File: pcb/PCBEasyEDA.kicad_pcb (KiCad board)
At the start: 2 copper layers, 63.4 x 89 mm, 56 parts

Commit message: YAY
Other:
- board text removed: "#10: Error: unsupported layer id: 100 found in CIRCLE (gge2481) of gge9d629947a8bba335; circle ignored"
- board text removed: "#11: Error: unsupported layer id: 100 found in CIRCLE (gge2484) of gge9d629947a8bba335; circle ignored"
- board text removed: "#12: Error: unsupported layer id: 100 found in CIRCLE (gge2487) of gge9d629947a8bba335; circle ignored"
- board text removed: "#13: Error: unsupported layer id: 100 found in CIRCLE (gge2490) of gge9d629947a8bba335; circle ignored"
- board text removed: "#14: Error: unsupported layer id: 100 found in CIRCLE (gge2493) of gge9d629947a8bba335; circle ignored"
- board text removed: "#15: Error: unsupported layer id: 100 found in CIRCLE (gge2496) of gge9d629947a8bba335; circle ignored"
- board text removed: "#16: Error: unsupported layer id: 100 found in CIRCLE (gge2499) of gge9d629947a8bba335; circle ignored"
- board text removed: "#17: Error: unsupported layer id: 100 found in CIRCLE (gge2502) of gge9d629947a8bba335; circle ignored"
- board text removed: "#18: Error: unsupported layer id: 100 found in CIRCLE (gge2505) of gge9d629947a8bba335; circle ignored"
- board text removed: "#19: Error: unsupported layer id: 100 found in CIRCLE (gge2508) of gge9d629947a8bba335; circle ignored"
- board text removed: "#1: Info: below are the conversion remarks. The conversion may contain errors. Please read the remarks carefully and run the DRC check to solve issues. To find a component mentioned in the remarks go to: Kicad menu Edit > Find and enter the EDA_id (gge....); search for other text items. Only the id of the footprint can be found; the id of the shape is in the input json. You can export the footpri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"
- board text removed: "#20: Error: unsupported layer id: 100 found in CIRCLE (gge2511) of gge9d629947a8bba335; circle ignored"
- board text removed: "#21: Error: unsupported layer id: 100 found in CIRCLE (gge2514) of gge9d629947a8bba335; circle ignored"
- board text removed: "#22: Error: unsupported layer id: 100 found in CIRCLE (gge2517) of gge9d629947a8bba335; circle ignored"
- board text removed: "#23: Error: unsupported layer id: 100 found in CIRCLE (gge2520) of gge9d629947a8bba335; circle ignored"
- board text removed: "#24: Error: unsupported layer id: 100 found in CIRCLE (gge2523) of gge9d629947a8bba335; circle ignored"
- board text removed: "#25: Error: unsupported layer id: 100 found in CIRCLE (gge2526) of gge9d629947a8bba335; circle ignored"
- board text removed: "#26: Error: unsupported layer id: 100 found in CIRCLE (gge2529) of gge9d629947a8bba335; circle ignored"
- board text removed: "#27: Error: unsupported layer id: 100 found in CIRCLE (gge2532) of gge9d629947a8bba335; circle ignored"
- board text removed: "#28: Error: unsupported layer id: 100 found in CIRCLE (gge2535) of gge9d629947a8bba335; circle ignored"
- board text removed: "#29: Error: unsupported layer id: 100 found in CIRCLE (gge2538) of gge9d629947a8bba335; circle ignored"
- board text removed: "#30: Error: unsupported layer id: 100 found in CIRCLE (gge2541) of gge9d629947a8bba335; circle ignored"
- board text removed: "#31: Error: unsupported layer id: 100 found in CIRCLE (gge2544) of gge9d629947a8bba335; circle ignored"
- board text removed: "#32: Error: unsupported layer id: 100 found in CIRCLE (gge2547) of gge9d629947a8bba335; circle ignored"
- board text removed: "#33: Error: unsupported layer id: 100 found in CIRCLE (gge2550) of gge9d629947a8bba335; circle ignored"
- board text removed: "#34: Error: unsupported layer id: 100 found in CIRCLE (gge2553) of gge9d629947a8bba335; circle ignored"
- board text removed: "#35: Error: unsupported layer id: 99 found in SOLIDREGION (gge2556) of gge9d629947a8bba335; solidregion ignored"
- board text removed: "#36: Error: unsupported layer id: 101 found in CIRCLE (gge3858) of gge6f41a13c46c13e35; circle ignored"
- board text removed: "#37: Error: unsupported layer id: 100 found in SOLIDREGION (gge3861) of gge6f41a13c46c13e35; solidregion ignored"
- board text removed: "#38: Error: unsupported layer id: 100 found in SOLIDREGION (gge3864) of gge6f41a13c46c13e35; solidregion ignored"
- board text removed: "#39: Error: unsupported layer id: 100 found in SOLIDREGION (gge3867) of gge6f41a13c46c13e35; solidregion ignored"
- board text removed: "#40: Error: unsupported layer id: 99 found in SOLIDREGION (gge3870) of gge6f41a13c46c13e35; solidregion ignored"
- board text removed: "#41: Error: unsupported layer id: 101 found in CIRCLE (gge3957) of ggee70bf5162dc4a40a; circle ignored"
- board text removed: "#42: Error: unsupported layer id: 100 found in SOLIDREGION (gge3960) of ggee70bf5162dc4a40a; solidregion ignored"
- board text removed: "#43: Error: unsupported layer id: 100 found in SOLIDREGION (gge3963) of ggee70bf5162dc4a40a; solidregion ignored"
- board text removed: "#44: Error: unsupported layer id: 100 found in SOLIDREGION (gge3966) of ggee70bf5162dc4a40a; solidregion ignored"
- board text removed: "#45: Error: unsupported layer id: 99 found in SOLIDREGION (gge3969) of ggee70bf5162dc4a40a; solidregion ignored"
- board text removed: "#46: Error: unsupported layer id: 101 found in CIRCLE (gge4056) of ggedc7a9a5c0e95c560; circle ignored"
- board text removed: "#47: Error: unsupported layer id: 100 found in SOLIDREGION (gge4059) of ggedc7a9a5c0e95c560; solidregion ignored"
- board text removed: "#48: Error: unsupported layer id: 100 found in SOLIDREGION (gge4062) of ggedc7a9a5c0e95c560; solidregion ignored"
- board text removed: "#49: Error: unsupported layer id: 100 found in SOLIDREGION (gge4065) of ggedc7a9a5c0e95c560; solidregion ignored"
- board text removed: "#4: Error: unsupported layer id: 101 found in CIRCLE (gge2463) of gge9d629947a8bba335; circle ignored"
- board text removed: "#50: Error: unsupported layer id: 99 found in SOLIDREGION (gge4068) of ggedc7a9a5c0e95c560; solidregion ignored"
- board text removed: "#51: Error: unsupported layer id: 101 found in CIRCLE (gge4155) of ggefb7ad87a757e0b06; circle ignored"
- board text removed: "#52: Error: unsupported layer id: 100 found in SOLIDREGION (gge4158) of ggefb7ad87a757e0b06; solidregion ignored"
- board text removed: "#53: Error: unsupported layer id: 100 found in SOLIDREGION (gge4161) of ggefb7ad87a757e0b06; solidregion ignored"
- board text removed: "#54: Error: unsupported layer id: 100 found in SOLIDREGION (gge4164) of ggefb7ad87a757e0b06; solidregion ignored"
- board text removed: "#55: Error: unsupported layer id: 99 found in SOLIDREGION (gge4167) of ggefb7ad87a757e0b06; solidregion ignored"
- board text removed: "#56: Error: unsupported layer id: 101 found in CIRCLE (gge4254) of ggec2f152703e6b9492; circle ignored"
- board text removed: "#57: Error: unsupported layer id: 100 found in SOLIDREGION (gge4257) of ggec2f152703e6b9492; solidregion ignored"
- board text removed: "#58: Error: unsupported layer id: 100 found in SOLIDREGION (gge4260) of ggec2f152703e6b9492; solidregion ignored"
- board text removed: "#59: Error: unsupported layer id: 100 found in SOLIDREGION (gge4263) of ggec2f152703e6b9492; solidregion ignored"
- board text removed: "#5: Error: unsupported layer id: 100 found in CIRCLE (gge2466) of gge9d629947a8bba335; circle ignored"
- board text removed: "#60: Error: unsupported layer id: 99 found in SOLIDREGION (gge4266) of ggec2f152703e6b9492; solidregion ignored"
- board text removed: "#61: Error: unsupported layer id: 101 found in CIRCLE (gge4353) of gge384a2c6d2d577bb5; circle ignored"
- board text removed: "#62: Error: unsupported layer id: 100 found in SOLIDREGION (gge4356) of gge384a2c6d2d577bb5; solidregion ignored"
- board text removed: "#63: Error: unsupported layer id: 100 found in SOLIDREGION (gge4359) of gge384a2c6d2d577bb5; solidregion ignored"
- board text removed: "#64: Error: unsupported layer id: 100 found in SOLIDREGION (gge4362) of gge384a2c6d2d577bb5; solidregion ignored"
- board text removed: "#65: Error: unsupported layer id: 99 found in SOLIDREGION (gge4365) of gge384a2c6d2d577bb5; solidregion ignored"
- board text removed: "#66: Error: unsupported layer id: 101 found in CIRCLE (gge4452) of ggecd7fe670e50dd6fe; circle ignored"
- board text removed: "#67: Error: unsupported layer id: 100 found in SOLIDREGION (gge4455) of ggecd7fe670e50dd6fe; solidregion ignored"
- board text removed: "#68: Error: unsupported layer id: 100 found in SOLIDREGION (gge4458) of ggecd7fe670e50dd6fe; solidregion ignored"
- board text removed: "#69: Error: unsupported layer id: 100 found in SOLIDREGION (gge4461) of ggecd7fe670e50dd6fe; solidregion ignored"
- board text removed: "#6: Error: unsupported layer id: 100 found in CIRCLE (gge2469) of gge9d629947a8bba335; circle ignored"
- board text removed: "#70: Error: unsupported layer id: 99 found in SOLIDREGION (gge4464) of ggecd7fe670e50dd6fe; solidregion ignored"
- board text removed: "#71: Error: unsupported layer id: 101 found in CIRCLE (gge4551) of gge274f8fc57fc47f2d; circle ignored"
- board text removed: "#72: Error: unsupported layer id: 100 found in SOLIDREGION (gge4554) of gge274f8fc57fc47f2d; solidregion ignored"
- board text removed: "#73: Error: unsupported layer id: 100 found in SOLIDREGION (gge4557) of gge274f8fc57fc47f2d; solidregion ignored"
- board text removed: "#74: Error: unsupported layer id: 100 found in SOLIDREGION (gge4560) of gge274f8fc57fc47f2d; solidregion ignored"
- board text removed: "#75: Error: unsupported layer id: 99 found in SOLIDREGION (gge4563) of gge274f8fc57fc47f2d; solidregion ignored"
- board text removed: "#7: Error: unsupported layer id: 100 found in CIRCLE (gge2472) of gge9d629947a8bba335; circle ignored"
- board text removed: "#8: Error: unsupported layer id: 100 found in CIRCLE (gge2475) of gge9d629947a8bba335; circle ignored"
- board text removed: "#9: Error: unsupported layer id: 100 found in CIRCLE (gge2478) of gge9d629947a8bba335; circle ignored"

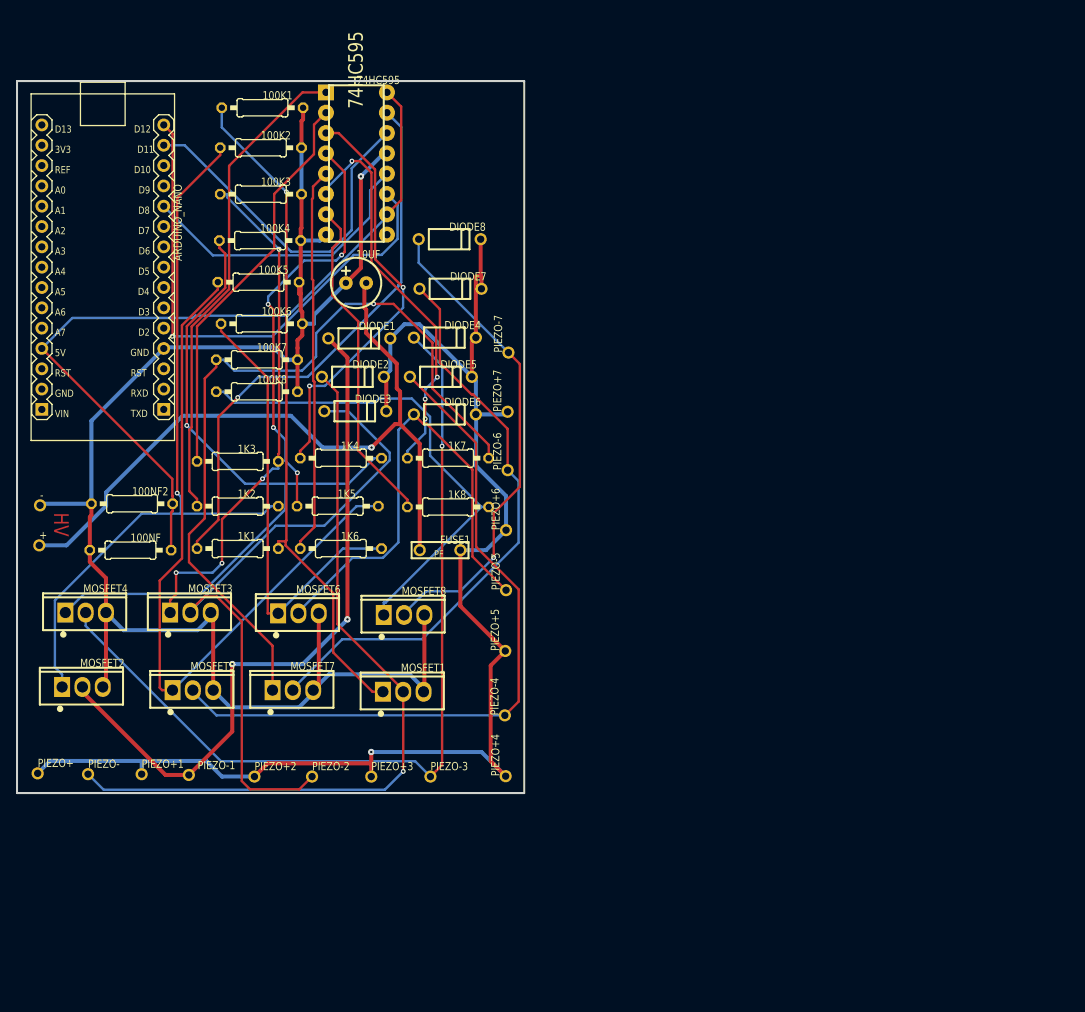
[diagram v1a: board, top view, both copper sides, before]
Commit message: e
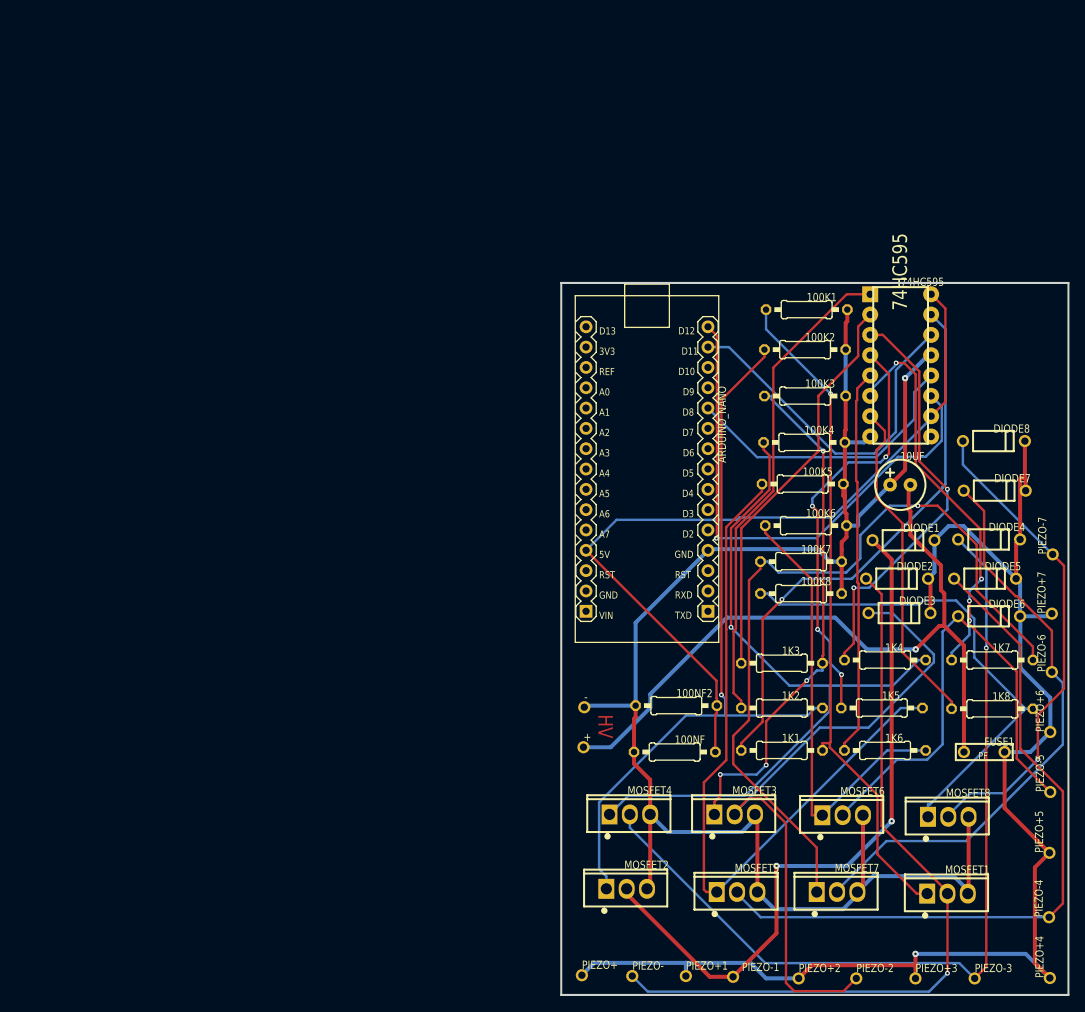
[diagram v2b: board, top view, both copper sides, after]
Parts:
- moved 100K1 72.6 mm to (124.8, 51.5)
- moved 100K5 72.6 mm to (124.3, 73.3)
- moved 100NF 72.6 mm to (108.3, 106.8)
- moved 74HC595 72.6 mm to (142.9, 69.9)
- moved MOSFET1 72.6 mm to (142.4, 124.5)
- moved MOSFET2 72.6 mm to (102.3, 123.9)
- moved MOSFET3 72.6 mm to (115.8, 114.6)
- moved PIEZO+2 72.6 mm to (123.8, 135.1)
- moved PIEZO+3 72.6 mm to (138.4, 135.1)
- moved PIEZO+5 72.6 mm to (155.1, 119.4)
- moved PIEZO-2 72.6 mm to (131.0, 135.1)
- moved + 72.6 mm to (96.9, 106.2)
- moved 100K2 72.6 mm to (124.6, 56.5)
- moved 100K3 72.6 mm to (124.6, 62.3)
- moved 100K7 72.6 mm to (124.1, 83.0)
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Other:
- board text added: "ok"
